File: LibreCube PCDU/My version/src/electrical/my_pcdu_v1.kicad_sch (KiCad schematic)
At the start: 106 parts, among them J1 Conn_01x02, J2 Conn_01x02, J3 Conn_01x02, J4 Conn_01x02, J5 Conn_01x02, J6 Conn_01x02, J7 Conn_01x02, M1 MountingHole, M2 MountingHole, M3 MountingHole, M4 MountingHole, U1 TPS2034, U10 TPS2034, U11 TPS61032, U12 TPS61032, U2 TPS2034, U3 TPS2034, U4 TPS2034, U5 TPS61032, U6 TPS61032, U7 bq24002, U8 bq24002, U9 TPS2034

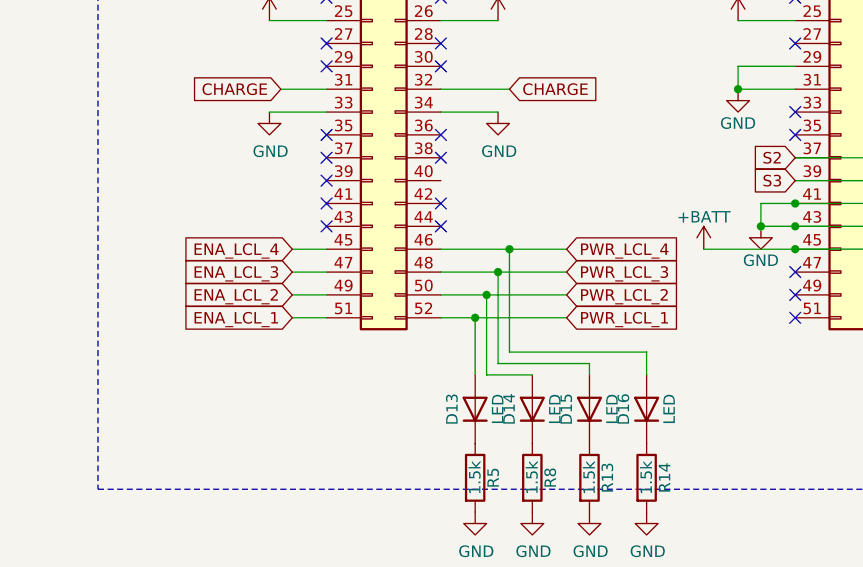
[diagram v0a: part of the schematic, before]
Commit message: Uploaded PCDUv2
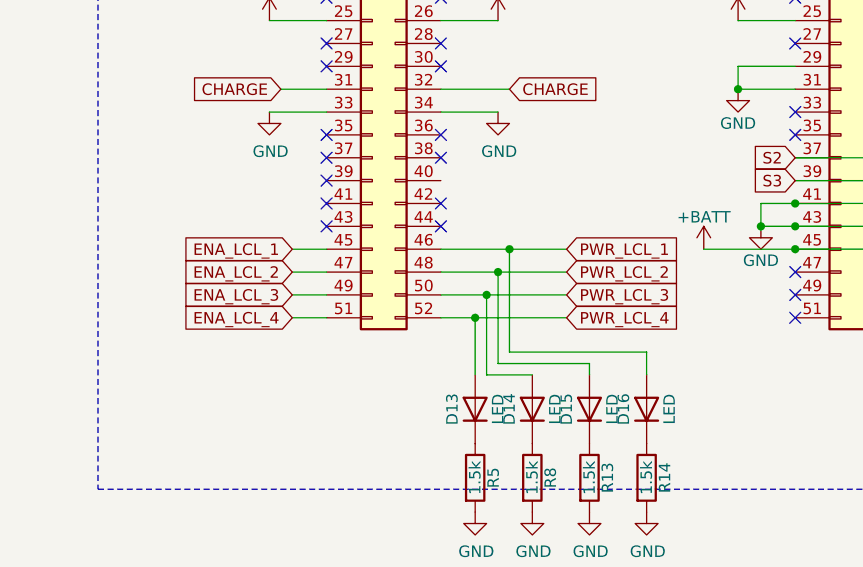
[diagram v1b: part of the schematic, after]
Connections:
- net ENA_LCL_1: now also H1.45 (Pin_45); no longer H1.51 (Pin_51)
- net ENA_LCL_2: now also H1.47 (Pin_47); no longer H1.49 (Pin_49)
- net ENA_LCL_3: now also H1.49 (Pin_49); no longer H1.47 (Pin_47)
- net ENA_LCL_4: now also H1.51 (Pin_51); no longer H1.45 (Pin_45)
- net PWR_LCL_1: now also D16.2 (A), H1.46 (Pin_46); no longer D13.2 (A), H1.52 (Pin_52)
- net PWR_LCL_2: now also D15.2 (A), H1.48 (Pin_48); no longer D14.2 (A), H1.50 (Pin_50)
- net PWR_LCL_3: now also D14.2 (A), H1.50 (Pin_50); no longer D15.2 (A), H1.48 (Pin_48)
- net PWR_LCL_4: now also D13.2 (A), H1.52 (Pin_52); no longer D16.2 (A), H1.46 (Pin_46)
